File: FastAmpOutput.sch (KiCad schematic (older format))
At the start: 20 parts

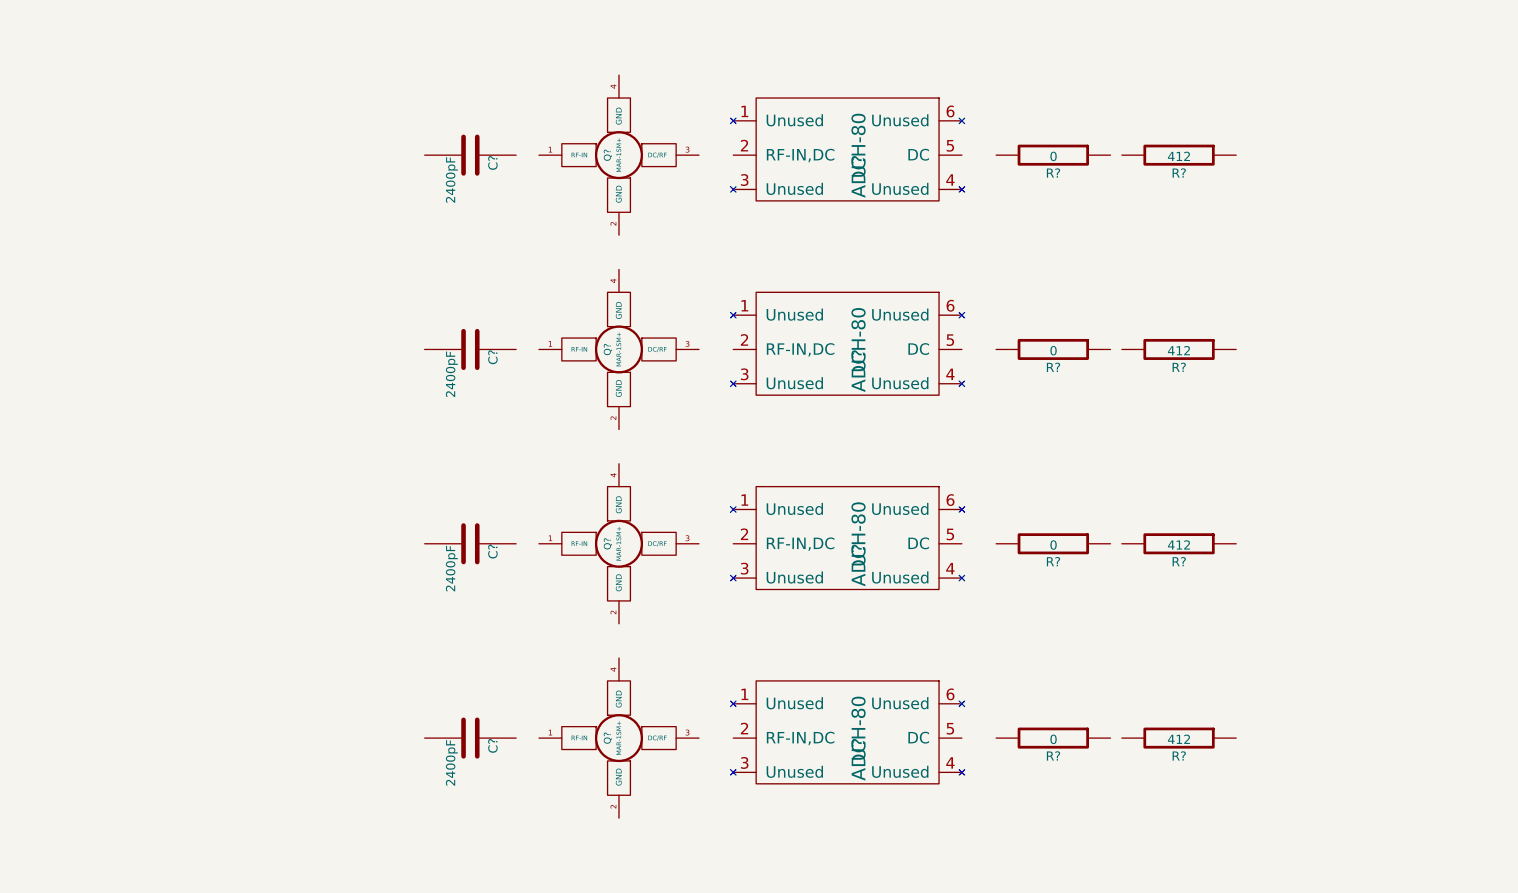
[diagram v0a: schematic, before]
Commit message: Schematic complete (mostly, may have bugs) initial layout of parts on pcb, no connecting bits
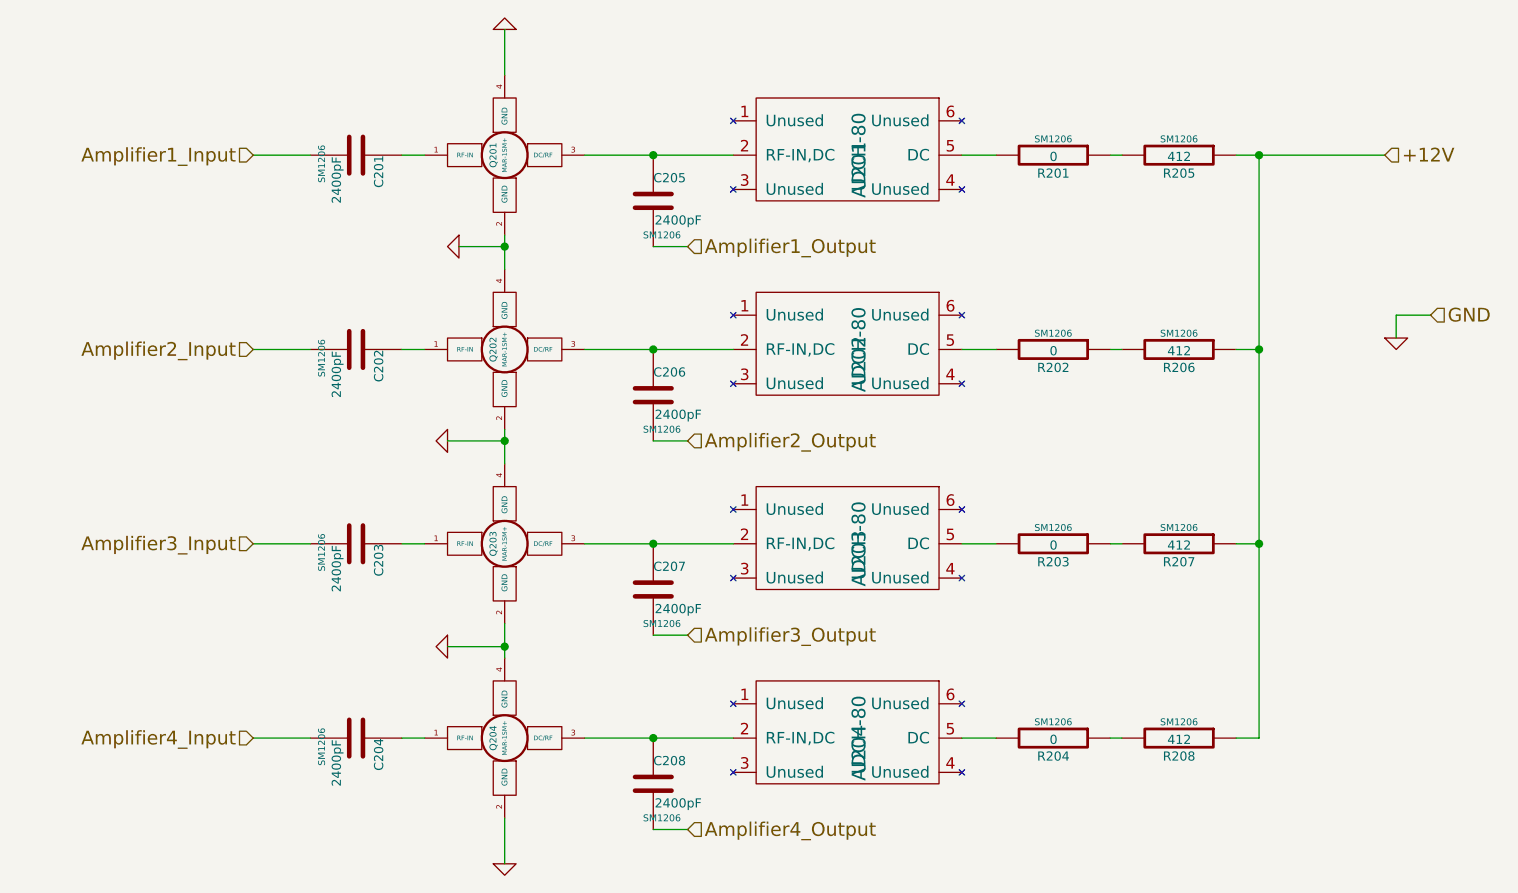
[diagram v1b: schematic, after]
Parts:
- added C205, C206, C207, C208: 2400pF, SM1206, symbol C
- C201, C202, C203, C204: renamed from C?; footprint ~ -> SM1206
- R201, R202, R203, R204, R205, R206, R207, R208: renamed from R?; footprint ~ -> SM1206
- gave numbers to parts that had none: 8
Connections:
- net +12V: now reaches R205.1
- net +12V: now also R206.1, R207.1, R208.1
- net at R205.2: now also R201.1
- net at R201.2: now also U201.5 (DC)
- net at U201.2 (RF-IN,DC): now also Q201.3 (DC/RF), C205.1
- net at Q201.1 (RF-IN): now also C201.1
- net GND: now reaches Q201.2 (GND)
- net GND: now also Q201.4 (GND), Q202.2 (GND), Q202.4 (GND), Q203.2 (GND), Q203.4 (GND), Q204.2 (GND), Q204.4 (GND)
- net Amplifier1_Input: now reaches C201.2
- net at R206.2: now also R202.1
- net at R202.2: now also U202.5 (DC)
- net at U202.2 (RF-IN,DC): now also Q202.3 (DC/RF), C206.1
- net at Q202.1 (RF-IN): now also C202.1
- net Amplifier2_Input: now reaches C202.2
- net at R207.2: now also R203.1
- net at R203.2: now also U203.5 (DC)
- net at U203.2 (RF-IN,DC): now also Q203.3 (DC/RF), C207.1
- net at Q203.1 (RF-IN): now also C203.1
- net Amplifier3_Input: now reaches C203.2
- net at R208.2: now also R204.1
- net at R204.2: now also U204.5 (DC)
- net at U204.2 (RF-IN,DC): now also Q204.3 (DC/RF), C208.1
- net at Q204.1 (RF-IN): now also C204.1
- net Amplifier4_Input: now reaches C204.2
- new net Amplifier1_Output: C205.2
- new net Amplifier2_Output: C206.2
- new net Amplifier3_Output: C207.2
- new net Amplifier4_Output: C208.2
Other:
- moved on the sheet: C201, C202, C203, C204, Q201, Q202, Q203, Q204
